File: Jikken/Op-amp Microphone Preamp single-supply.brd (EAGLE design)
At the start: 100 x 80 mm, 17 parts, among them IC1 AD822N

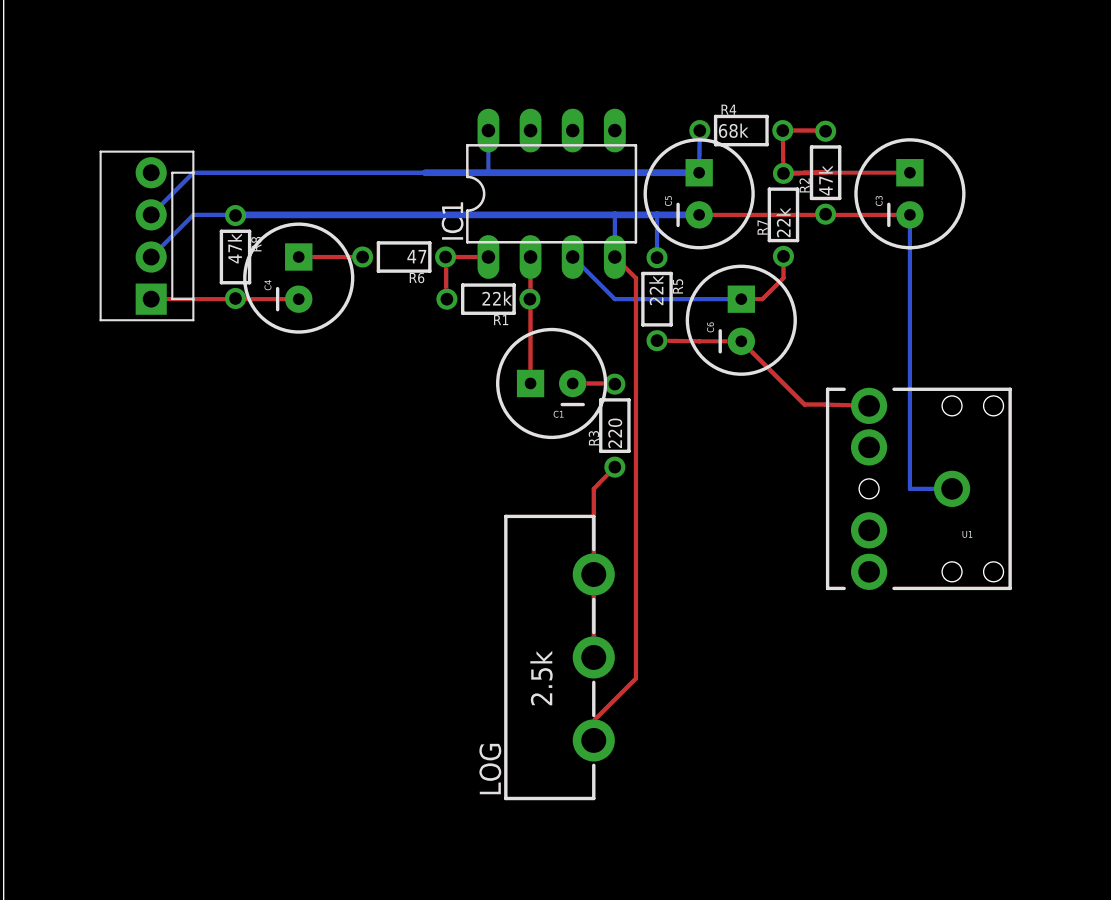
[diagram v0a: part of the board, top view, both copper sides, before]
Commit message: jikken amp
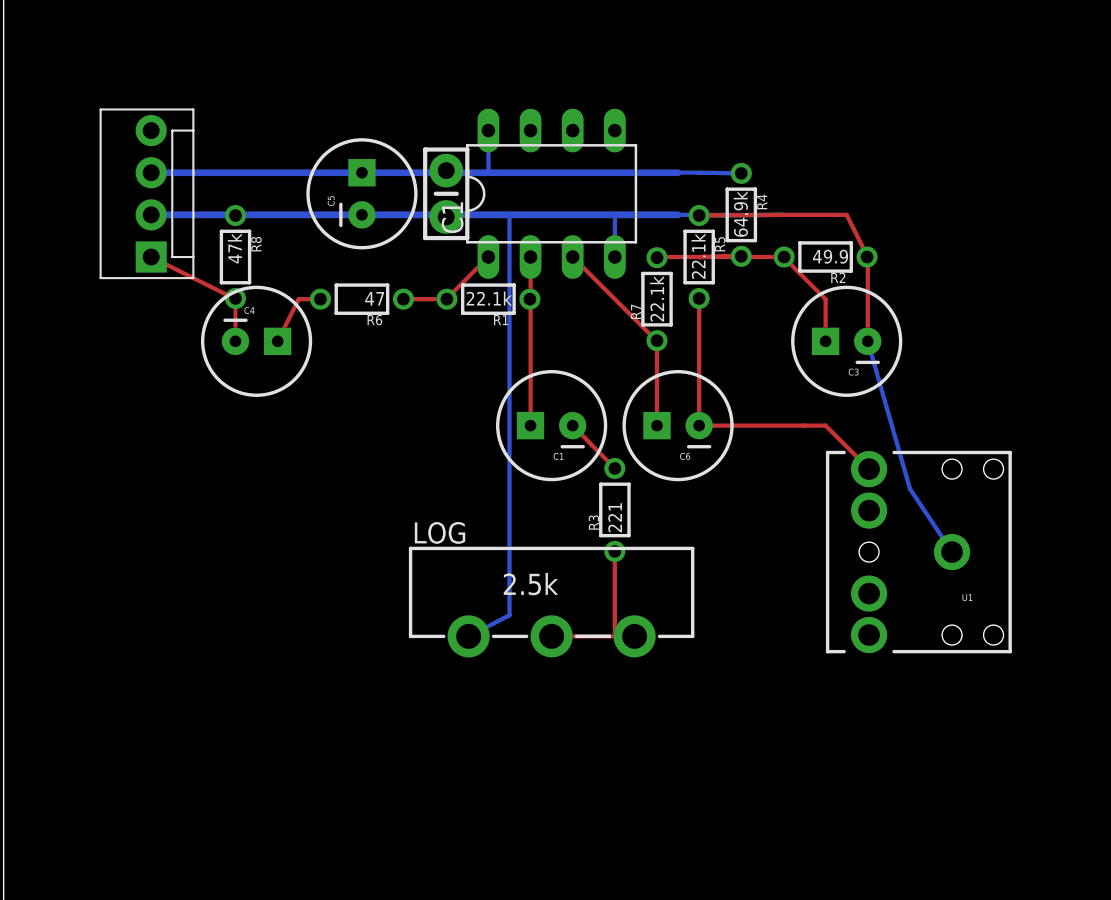
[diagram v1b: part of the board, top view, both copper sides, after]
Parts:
- added C2: 0.1uF, SparkFun:CAP-PTH-SMALL-KIT
- C1, C4: value 100u -> 100uF/25V
- R1, R5, R7: value 22k -> 22.1k
- R2: value 47k -> 49.9
- R3: value 220 -> 221
- R4: value 68k -> 64.9k
- moved C5 20.3 mm to (21.6, 49.5)
- moved C3 9.67 mm to (50.8, 40.6), turned to 180 degrees
- moved R7 9.16 mm to (39.4, 43.2)
- moved C6 7.41 mm to (40.6, 35.6), turned to 180 degrees
- moved R4 5.08 mm to (44.5, 48.3), turned to 270 degrees
- moved R3 5.08 mm to (36.8, 30.5)
- moved R2 5.08 mm to (49.5, 45.7), turned to 180 degrees
- moved C4 4.58 mm to (15.2, 40.6), turned to 0 degrees
- moved U1 3.81 mm to (57.1, 27.9)
- moved R5 3.59 mm to (41.9, 45.7)
- moved R6 3.59 mm to (21.6, 43.2)
- moved LOG 2.84 mm to (33.0, 22.9), turned to 0 degrees
- moved C1 2.54 mm to (33.0, 35.6)
- moved JP2 2.54 mm to (8.89, 45.7)
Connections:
- net GND: now also C2.2
- net VCC: now also C2.1
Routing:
- net N$8: track 14.4 -> 19.0 mm
- net N$6: track 15.6 -> 12.3 mm
- net N$5: track 7.70 -> 10.2 mm
- net GND: track 101.8 -> 103.5 mm
- net N$1: track 17.9 -> 19.0 mm
- net N$3: track 5.20 -> 6.25 mm
- net N$2: track 2.58 -> 3.62 mm
- net VCC: track 39.2 -> 38.2 mm
- net N$4: track 12.0 -> 11.3 mm
- net N$13: track 8.97 -> 8.30 mm
